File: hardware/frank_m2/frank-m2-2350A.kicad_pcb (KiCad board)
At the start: 2 copper layers, 88.9 x 50.8 mm, 124 parts, among them J1 Audio Jumpers, J2 PWM Jumper, P1 Power (+5V), Q1 BC850, Q2 BC850, Q3 BC850, Q4 BC850, SW1 Reset, SW2 Boot, U1 NCP1117 3.3, U2 RP2350A, U3 ESP-PSRAM32, U4 W25Q128JVSQ, U5 TDA1387T, Y1 ABM8-272-T3 12 MHz

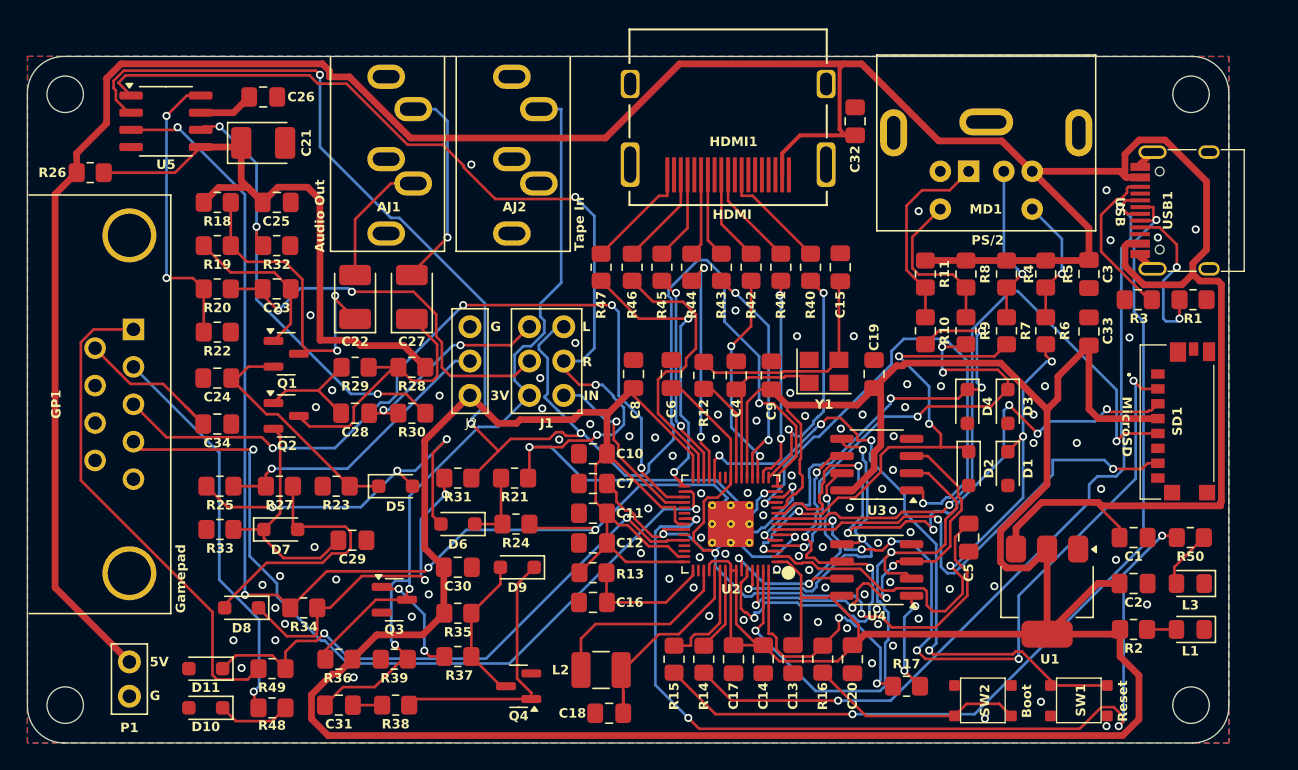
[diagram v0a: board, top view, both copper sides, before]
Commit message: HW Rev 1.01
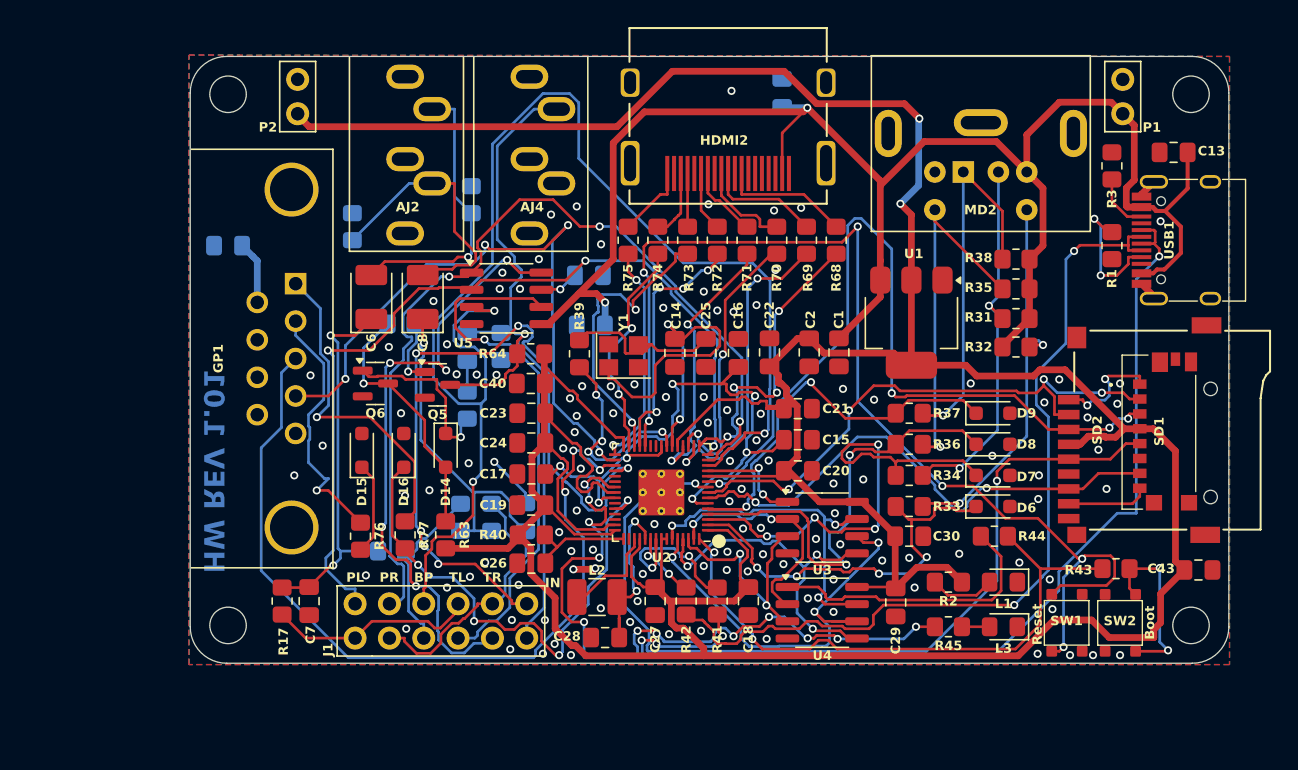
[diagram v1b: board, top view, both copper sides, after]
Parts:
- removed AJ1: PJ-325C, FRANK:Jack (3.5mm)
- removed C10, C11, C12, C31, C32, C33, C34, C5: 100n, FRANK:Capacitor (0805)
- removed D1, D10, D11, D2, D3, D4: 3V3, FRANK:Diode (SOD-323)
- removed D5: 1N4148, FRANK:Diode (SOD-323)
- removed HDMI1: HDMI Female, FRANK:HDMI (female)
- removed J2: PWM Jumper, FRANK:Pin Header (1x03)
- removed MD1: Mini-DIN-6, FRANK:MiniDIN (6 Pin, female)
- removed Q1, Q2, Q3, Q4: BC850, FRANK:SOT-23
- removed R10, R23, R6, R7, R9: 100R, FRANK:Resistor (0805)
- removed R11: 1k, FRANK:Resistor (0805)
- removed R12, R16, R28, R4, R48, R49, R5, R50, R8: 1K, FRANK:Resistor (0805)
- removed R13: 33R, FRANK:Resistor (0805)
- removed R14, R15: 27R, FRANK:Resistor (0805)
- removed R24, R25, R27: 200R, FRANK:Resistor (0805)
- removed R26: 10R, FRANK:Resistor (0805)
- removed R29: 100K, FRANK:Resistor (0805)
- removed R30: 20K, FRANK:Resistor (0805)
- removed R46, R47: 270R, FRANK:Resistor (0805)
- added AJ4: PJ-325C, FRANK:Jack (3.5mm), F.Cu at (166.1, 65.7)
- added C40: 100n, FRANK:Capacitor (0805), F.Cu at (166.2, 88.4)
- added C41: 100n, FRANK:Capacitor (0805), B.Cu at (161.5, 85.7)
- added C42: 100n, FRANK:Capacitor (0805), B.Cu at (184.8, 66.9)
- added C43: 100n, FRANK:Capacitor (0805), F.Cu at (215.6, 102.2)
- added C44: 100n, FRANK:Capacitor (0805), B.Cu at (143.8, 78.2)
- added D14: 1N4148, FRANK:Diode (SOD-323), F.Cu at (159.9, 93.3)
- added D15: 3V3, FRANK:Diode (SOD-323), F.Cu at (153.7, 93.3)
- added D16: 3V3, FRANK:Diode (SOD-323), F.Cu at (156.8, 93.3)
- added HDMI2: HDMI Female, FRANK:HDMI (female), F.Cu at (180.8, 72.1)
- added MD2: Mini-DIN-6, FRANK:MiniDIN (6 Pin, female), F.Cu at (198.2, 72.8)
- added P2: Power (+3.3V), FRANK:Pin Header (1x02), F.Cu at (148.9, 65.9)
- added Q5: BC850, FRANK:SOT-23, F.Cu at (159.3, 88.5)
- added Q6: BC850, FRANK:SOT-23, F.Cu at (154.7, 88.4)
- added R63: 10K, FRANK:Resistor (0805), F.Cu at (159.9, 99.6)
- added R64: 1K, FRANK:Resistor (0805), F.Cu at (166.2, 86.2)
- added R65: 10K, FRANK:Resistor (0805), B.Cu at (156.6, 84.0)
- added R66: 10K, FRANK:Resistor (0805), B.Cu at (161.5, 90.0)
- added R67: 100R, FRANK:Resistor (0805), B.Cu at (164.0, 85.7)
- added R68: 270R, FRANK:Resistor (0805), F.Cu at (188.8, 77.8)
- added R69: 270R, FRANK:Resistor (0805), F.Cu at (186.6, 77.8)
- added R70: 270R, FRANK:Resistor (0805), F.Cu at (184.4, 77.8)
- added R71: 270R, FRANK:Resistor (0805), F.Cu at (182.2, 77.8)
- added R72: 270R, FRANK:Resistor (0805), F.Cu at (180.0, 77.8)
- added R73: 270R, FRANK:Resistor (0805), F.Cu at (177.8, 77.8)
- added R74: 270R, FRANK:Resistor (0805), F.Cu at (175.6, 77.8)
- added R75: 270R, FRANK:Resistor (0805), F.Cu at (173.4, 77.8)
- added R76: 1K, FRANK:Resistor (0805), F.Cu at (153.6, 99.7)
- added R77: 1K, FRANK:Resistor (0805), F.Cu at (156.9, 99.6)
- added SD2: 104031-0811, FRANK:MicroSD (SMD, long), F.Cu at (205.2, 91.8)
- AJ2: value PJ-325C -> SJ1-353XNG
- C13: value 100n -> 10u
- C14, C25: value 100n -> 15p
- C15: value 15p -> 100n
- C17, C18: value 4.7u -> 100n
- C21, C22: value 10u -> 100n; footprint FRANK:Capacitor (3528, tantalum, polar) -> FRANK:Capacitor (0805)
- C23: value 1u -> 100n
- C26, C28: value 1u -> 4.7u
- C27: value 10u -> 4.7u; footprint FRANK:Capacitor (3528, tantalum, polar) -> FRANK:Capacitor (0805)
- C3: value 10u -> 1u; moved to B.Cu
- C4: value 15p -> 47u; moved to B.Cu
- C6: value 4.7u -> 10u; footprint FRANK:Capacitor (0805) -> FRANK:Capacitor (3528, tantalum, polar)
- C7: value 100n -> 10n
- C8: value 100n -> 10u; footprint FRANK:Capacitor (0805) -> FRANK:Capacitor (3528, tantalum, polar)
- C9: value 100n -> 10n; moved to B.Cu
- D6, D7, D8, D9: value 1N4148 -> 3V3
- J1: value Audio Jumpers -> Pin Header 2x18; footprint FRANK:Pin Header (2x03) -> FRANK:Pin Header (2x06)
- R17: value 0R -> 1K
- R18, R22: value 1K -> 330R; moved to B.Cu
- R19: value 100K -> 2K; moved to B.Cu
- R20: value 20K -> 2K; moved to B.Cu
- R21: value 51R -> 1K; moved to B.Cu
- R31: value 51R -> 1K
- R33: value 100 -> 100R
- R34: value 200R -> 100R
- R35: value 10K -> 1K
- R36: value 1K -> 100R
- R37: value 10K -> 100R
- R38: value 10K -> 1k
- R39: value 100R -> 1K
- R40: value 270R -> 33R
- R41, R42: value 270R -> 27R
- R43, R45: value 270R -> 1K
- R44: value 270R -> 0R
- moved P1 86.5 mm to (210.0, 65.9), turned to 0 degrees
- moved D8 56.9 mm to (200.4, 92.9), turned to 0 degrees
- moved R38 56.5 mm to (202.1, 79.2), turned to 180 degrees
- moved R32 55.2 mm to (202.1, 85.7)
- moved D7 52.9 mm to (200.4, 95.2)
- moved R33 51.0 mm to (194.2, 97.5)
- moved R35 47.8 mm to (202.1, 81.4), turned to 180 degrees
- moved C13 46.9 mm to (213.8, 71.3), turned to 180 degrees
- moved R17 46.6 mm to (147.8, 104.5), turned to -90 degrees
- moved R34 45.9 mm to (194.2, 95.2)
- moved R36 45.1 mm to (194.2, 92.9)
- moved C21 44.2 mm to (186.0, 90.3)
- moved R31 43.0 mm to (202.1, 83.6), turned to 180 degrees
- moved C29 40.5 mm to (193.2, 104.6), turned to -90 degrees
- moved C26 39.8 mm to (166.2, 101.7), turned to 180 degrees
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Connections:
- AJ2 pad R: unconnected-(AJ2-PadR) -> /Audio Out/R
- AJ2 pad RN: unconnected-(AJ2-PadRN) -> /Audio Out/R*
- AJ2 pad T: /LOAD_IN_D -> /Audio Out/L
- AJ2 pad TN: unconnected-(AJ2-PadTN) -> /Audio Out/L*
- C13 pad 1: +3V3 -> VBUS
- C14 pad 1: +3V3 -> /RP2350A/XIN
- C16 pad 1: /RP2350A/VREG_AVDD -> Net-(C15-Pad1)
- C17 pad 1: +3V3 -> Net-(C15-Pad1)
- C18 pad 1: Net-(U2-VREG_FB) -> +3V3
- C21 pad 1: /Audio Out/+5VA -> +3V3
- C22 pad 1: Net-(Q1-C) -> +3V3
- C22 pad 2: /Audio Out/R -> GND
- C23 pad 1: /RIGHT_OUT -> +3V3
- C23 pad 2: Net-(Q1-B) -> GND
- C24 pad 1: GND -> +3V3
- C24 pad 2: Net-(D5-K) -> GND
- C25 pad 1: /Audio Out/+5VA -> Net-(C25-Pad1)
- C26 pad 1: Net-(U5-FLT) -> /RP2350A/VREG_AVDD
- C27 pad 1: Net-(Q2-C) -> +3V3
- C27 pad 2: /Audio Out/L -> GND
- C28 pad 1: /LEFT_OUT -> Net-(U2-VREG_FB)
- C28 pad 2: Net-(Q2-B) -> GND
- C29 pad 1: GND -> +3V3
- C29 pad 2: Net-(D7-K) -> GND
- C3 pad 1: VBUS -> Net-(U5-FLT)
- C4 pad 1: /RP2350A/XIN -> GND
- C4 pad 2: GND -> VBUS
- C6 pad 1: Net-(C5-Pad1) -> Net-(C6-Pad1)
- C6 pad 2: GND -> /Audio Out/L
- C7 pad 1: Net-(C5-Pad1) -> Net-(C6-Pad1)
- C8 pad 1: +3V3 -> Net-(C8-Pad1)
- C8 pad 2: GND -> /Audio Out/R
- C9 pad 1: +3V3 -> Net-(C8-Pad1)
- D6 pad 1: Net-(D6-K) -> /GPIO0
- D6 pad 2: Net-(D5-A) -> GND
- D7 pad 1: Net-(D7-K) -> /GPIO1
- D7 pad 2: Net-(D7-A) -> GND
- D8 pad 1: Net-(D8-K) -> /GPIO2
- D8 pad 2: Net-(D7-A) -> GND
- D9 pad 1: Net-(D9-K) -> /GPIO3
- D9 pad 2: Net-(D9-A) -> GND
- J1 pad 1: /LEFT_OUT -> /A_OUTL
- J1 pad 2: /RIGHT_OUT -> /GPIO11
- J1 pad 3: /LOAD_IN_D -> /A_OUTR
- J1 pad 4: /GPIO22 -> /GPIO10
- J1 pad 5: /GPIO10 -> /A_OUTB
- J1 pad 6: /GPIO11 -> /GPIO9
- R17 pad 1: /RP2350A/QSPI_SS -> Net-(C6-Pad1)
- R17 pad 2: /RP2350A/FLASH_SS -> /A_OUTL
- R18 pad 1: /Audio Out/+5VA -> /Audio Out/L
- R18 pad 2: Net-(Q1-C) -> GND
- R19 pad 1: Net-(Q1-B) -> Net-(C6-Pad1)
- R19 pad 2: Net-(Q1-C) -> /A_OUTB
- R20 pad 1: Net-(U5-A_RIGHT) -> Net-(C8-Pad1)
- R20 pad 2: /RIGHT_OUT -> /A_OUTB
- R21 pad 1: Net-(D6-K) -> Net-(C8-Pad1)
- R21 pad 2: /GPIO10 -> /A_OUTR
- R22 pad 1: Net-(U5-A_RIGHT) -> /Audio Out/R
- R31 pad 1: Net-(D8-K) -> VBUS
- R31 pad 2: /GPIO11 -> Net-(MD2-Pad2)
- R32 pad 1: Net-(U5-A_LEFT) -> VBUS
- R32 pad 2: GND -> Net-(MD2-Pad6)
- R33 pad 1: Net-(D7-K) -> Net-(MD2-Pad6)
- R33 pad 2: GND -> /GPIO0
- R34 pad 1: Net-(D8-K) -> Net-(MD2-Pad2)
- R34 pad 2: /GPIO9 -> /GPIO1
- R35 pad 1: +3V3 -> VBUS
- R35 pad 2: Net-(D9-A) -> /PS2/PS/2 CLK
- R36 pad 1: +3V3 -> /PS2/PS/2 CLK
- R36 pad 2: /LOAD_IN_D -> /GPIO2
- R37 pad 1: Net-(D9-A) -> /PS2/PS/2 DATA
- R37 pad 2: Net-(Q3-B) -> /GPIO3
- R38 pad 1: Net-(C31-Pad2) -> VBUS
- R38 pad 2: Net-(D9-K) -> /PS2/PS/2 DATA
- R39 pad 1: /LOAD_IN_D -> /RP2350A/XOUT
- R39 pad 2: GND -> Net-(C25-Pad1)
- R40 pad 1: Net-(HDMI1-CLKN) -> +3V3
- R40 pad 2: /GPIO12 -> /RP2350A/VREG_AVDD
- R41 pad 1: Net-(HDMI1-CLKP) -> /D+
- R41 pad 2: /GPIO13 -> Net-(U2-USB_DP)
- R42 pad 1: Net-(HDMI1-D0N) -> /D-
- R42 pad 2: /GPIO14 -> Net-(U2-USB_DM)
- R43 pad 1: Net-(HDMI1-D0P) -> /RP2350A/QSPI_SS
- R43 pad 2: /GPIO15 -> /RP2350A/~{USB_BOOT}
- R44 pad 1: Net-(HDMI1-D1N) -> /RP2350A/QSPI_SS
- R44 pad 2: /GPIO16 -> /RP2350A/FLASH_SS
- R45 pad 1: Net-(HDMI1-D1P) -> Net-(L3-A)
- R45 pad 2: /GPIO17 -> GPIO25
- U2 pad 23: Net-(C5-Pad1) -> Net-(C15-Pad1)
- U2 pad 39: Net-(C5-Pad1) -> Net-(C15-Pad1)
- U2 pad 6: Net-(C5-Pad1) -> Net-(C15-Pad1)
- U5 pad 5: /Audio Out/+5VA -> VBUS
- U5 pad 6: Net-(U5-A_LEFT) -> /A_TDAL
- U5 pad 8: Net-(U5-A_RIGHT) -> /A_TDAR
- Y1 pad 3: Net-(C15-Pad1) -> Net-(C25-Pad1)
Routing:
- net VBUS: track 230.8 -> 128.1 mm, vias 0 -> 2
- net Net-(C5-Pad1): track 70.7 -> 0.00 mm, vias 4 -> 0
- net /GPIO11: track 118.3 -> 63.9 mm, vias 4 -> 3
- net /A_TDAR: track 0.00 -> 45.8 mm, vias 0 -> 5
- net /Audio Out/+5VA: track 45.1 -> 0.00 mm
- net /GPIO22: track 13.8 -> 56.0 mm, vias 1 -> 6
- net /A_TDAL: track 0.00 -> 39.3 mm, vias 0 -> 1
- net /RUN: track 48.1 -> 83.8 mm, vias 4 -> 6
- net Net-(U5-A_LEFT): track 33.0 -> 0.00 mm, vias 3 -> 0
- net Net-(C15-Pad1): track 16.4 -> 47.3 mm, vias 0 -> 7
- net /GPIO8: track 37.5 -> 7.98 mm
- net Net-(D5-A): track 29.1 -> 0.00 mm, vias 3 -> 0
- net Net-(MD2-Pad6): track 0.00 -> 28.5 mm, vias 0 -> 2
- net /RIGHT_OUT: track 28.5 -> 0.00 mm, vias 2 -> 0
- net Net-(C6-Pad1): track 0.00 -> 28.2 mm, vias 0 -> 2
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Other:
- board size 88.9 x 50.8 mm -> 76.8 x 44.9 mm
- board text added: "BP"
- board text added: "HW REV 1.01"
- board text added: "PL"
- board text added: "PR"
- board text added: "TL"
- board text added: "TR"
- board text added: "https://rh1.dev"
- board text removed: "3V"
- board text removed: "5V"
- board text removed: "Audio Out"
- board text removed: "G"
- board text removed: "Gamepad"
- board text removed: "HDMI"
- board text removed: "HW REV 1.0 https://rh1.dev"
- board text removed: "L"
- board text removed: "MicroSD"
- board text removed: "PS/2"
- board text removed: "R"
- board text removed: "Tape In"
- board text removed: "USB"
